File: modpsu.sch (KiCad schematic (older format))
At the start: 29 parts, among them J1 IN, J2 OUT, J3 IN, J4 OUT+, J5 OUT-, Q1 AO4805, Q2 12A

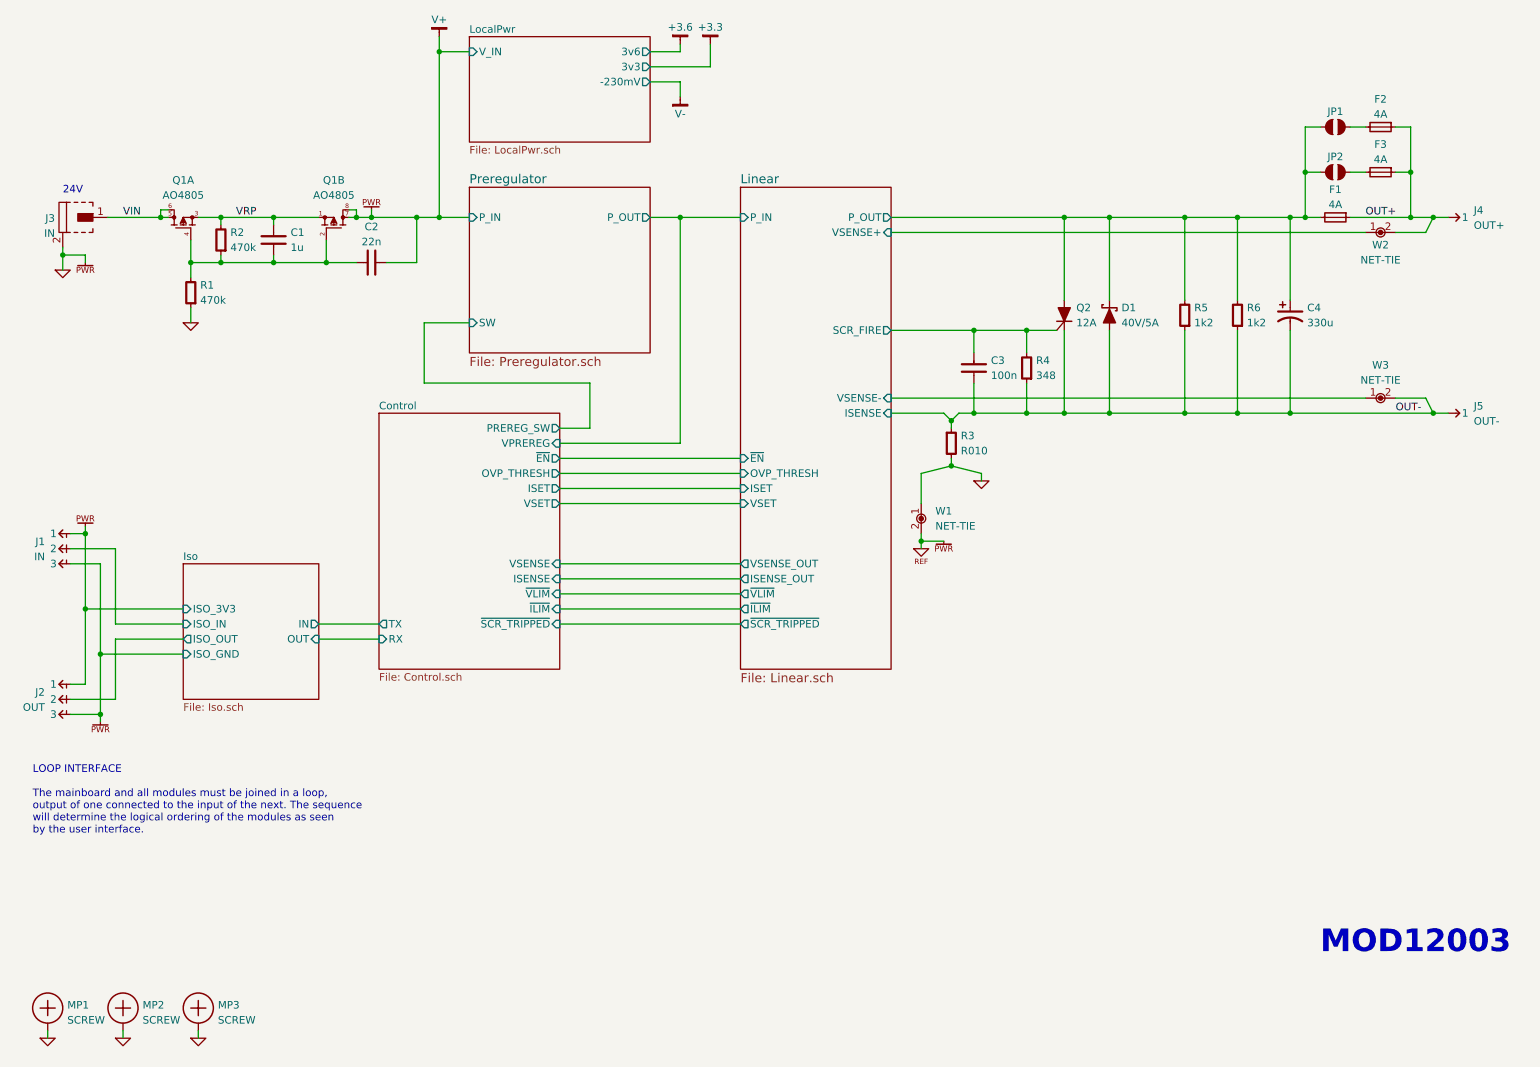
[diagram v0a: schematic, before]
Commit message: Piles and piles of work
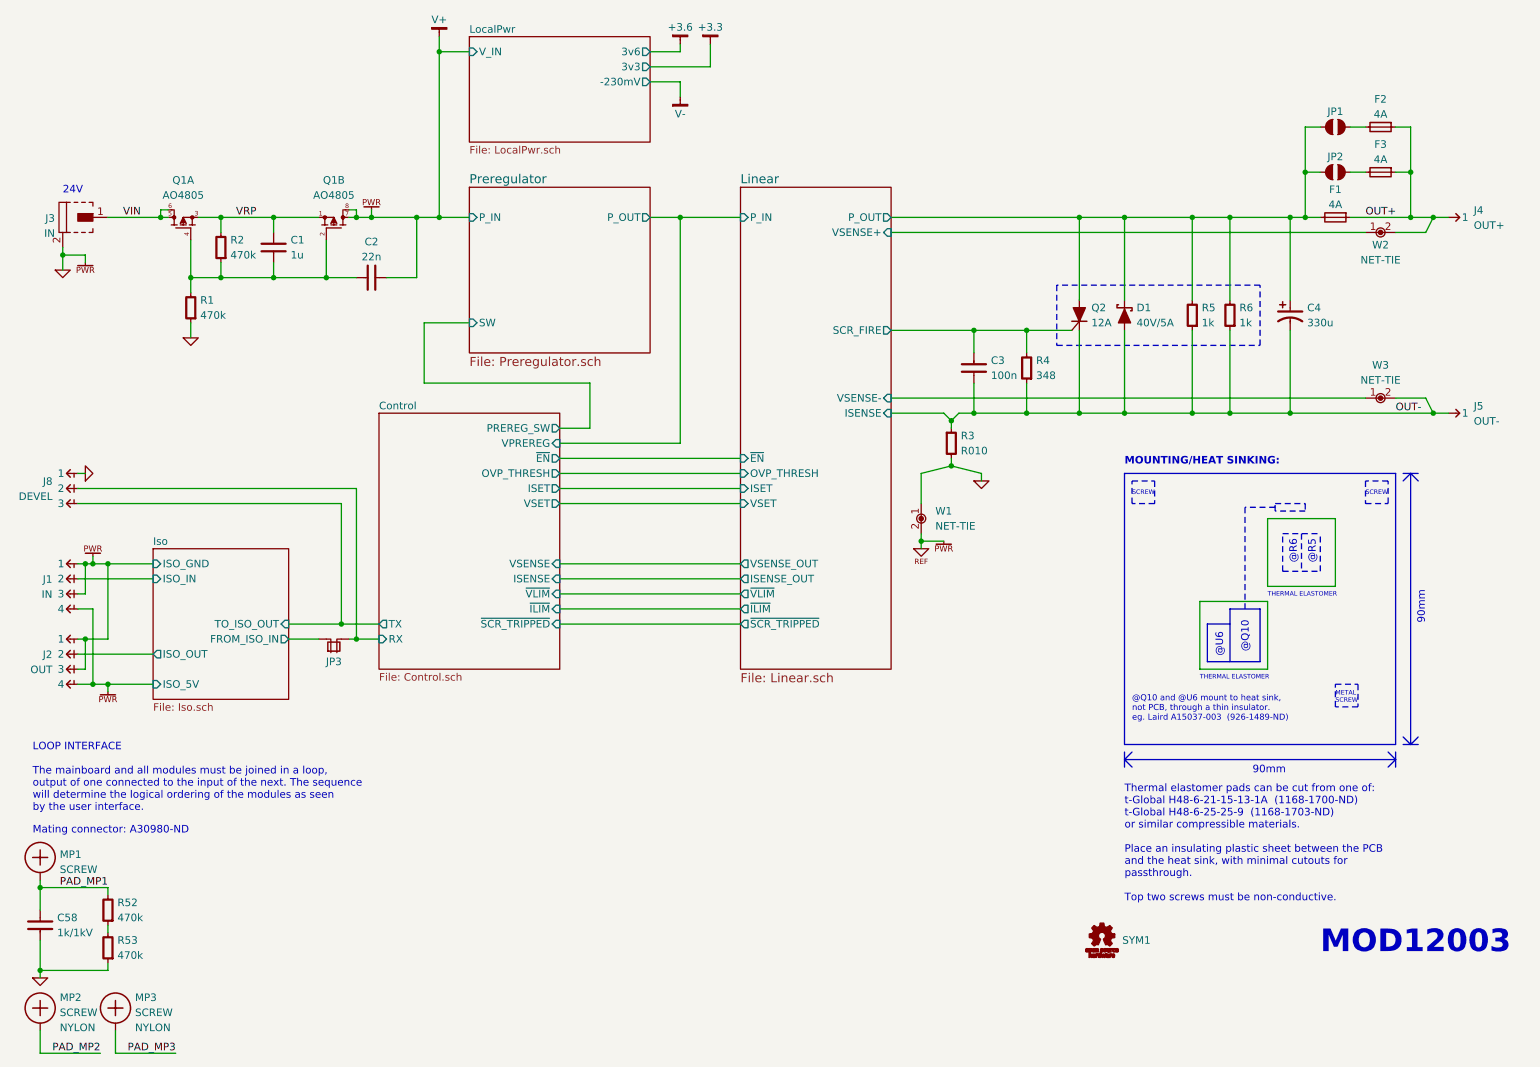
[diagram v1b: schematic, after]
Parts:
- removed J1: IN, conn-100mil:CONN-100MIL-M-1x3-SHROUD, symbol CONN-100MIL-M-1x3-SHROUD
- removed J2: OUT, conn-100mil:CONN-100MIL-M-1x3-SHROUD, symbol CONN-100MIL-M-1x3-SHROUD
- added C58: 1k/1kV, IPC7351-Nominal:CAPC3216X70, symbol C-1206
- added J1: IN, conn-100mil:CONN-100MIL-M-1x4-SHROUD, symbol CONN-100MIL-M-1x4-SHROUD
- added J2: OUT, conn-100mil:CONN-100MIL-M-1x4-SHROUD, symbol CONN-100MIL-M-1x4-SHROUD
- added J8: DEVEL, conn-100mil:CONN-100MIL-M-1x3, symbol CONN-100MIL-M-1x3
- added JP3: JUMPER, conn-100mil:CONN-100MIL-M-1x2, symbol JUMPER
- added R52, R53: 470k, IPC7351-Nominal:RESC1608X50, symbol R-0603
- added SYM1: OSHW-SCHEM-PCB6mm, mech:OSHW-6mm, symbol OSHW-SCHEM-PCB6mm
- F1, F2, F3: BOM DIST DIGIKEY 507-1193-2-ND -> DIST DIGIKEY 507-1193-1-ND
- MP2, MP3: Value2 (none) -> NYLON
- R5, R6: value 1k2 -> 1k; BOM RES SMD 1k2 5% [2512] -> RES SMD 1k [2512]
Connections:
- net Control/RX: now also J8.2, JP3.2
- net Control/TX: now also J8.3
- net GND: now also C58.2, J8.1, R53.1; no longer MP1.1, MP2.1, MP3.1
- net Iso/ISO_GND: now also J1.1, J1.3, J2.1, J2.3
- net Iso/ISO_IN: now also J1.2
- net Iso/ISO_OUT: now also J2.2
- new net: R52.1, R53.2
- new net Iso/FROM_ISO_IN: JP3.1
- new net Iso/ISO_5V: J1.4, J2.4
- new net PAD_MP1: C58.1, MP1.1, R52.2
- new net PAD_MP2: MP2.1
- new net PAD_MP3: MP3.1
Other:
- note added: "90mm"
- note added: "@Q10"
- note added: "@Q10 and @U6 mount to heat sink,\nnot PCB, through a thin insulator.\neg. Laird A15037-003 (926-1489-ND)"
- note added: "@R5"
- note added: "@R6"
- note added: "@U6"
- note added: "METAL\nSCREW"
- note added: "MOUNTING/HEAT SINKING:"
- note added: "Mating connector: A30980-ND"
- note added: "SCREW"
- note added: "THERMAL ELASTOMER"
- note added: "Thermal elastomer pads can be cut from one of:\nt-Global H48-6-21-15-13-1A (1168-1700-ND)\nt-Global H48-6-25-25-9 (1168-1703-ND)\nor similar compressible materials.\n\nPlace an insulating plastic sheet between the PCB\nand the heat sink, with minimal cutouts for\npassthrough.\n\nTop two screws must be non-conductive."
- moved on the sheet: C1, C2, D1, MP1, MP2, Q2, R1, R2, R5, R6
